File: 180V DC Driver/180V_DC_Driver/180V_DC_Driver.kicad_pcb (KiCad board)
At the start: 2 copper layers, 195 x 112 mm, 16 parts, among them J1 AC_In, J2 DC_Out, J3 Conn_01x02_Socket, J4 Conn_01x01_Socket, Q1 IRFP460PBF

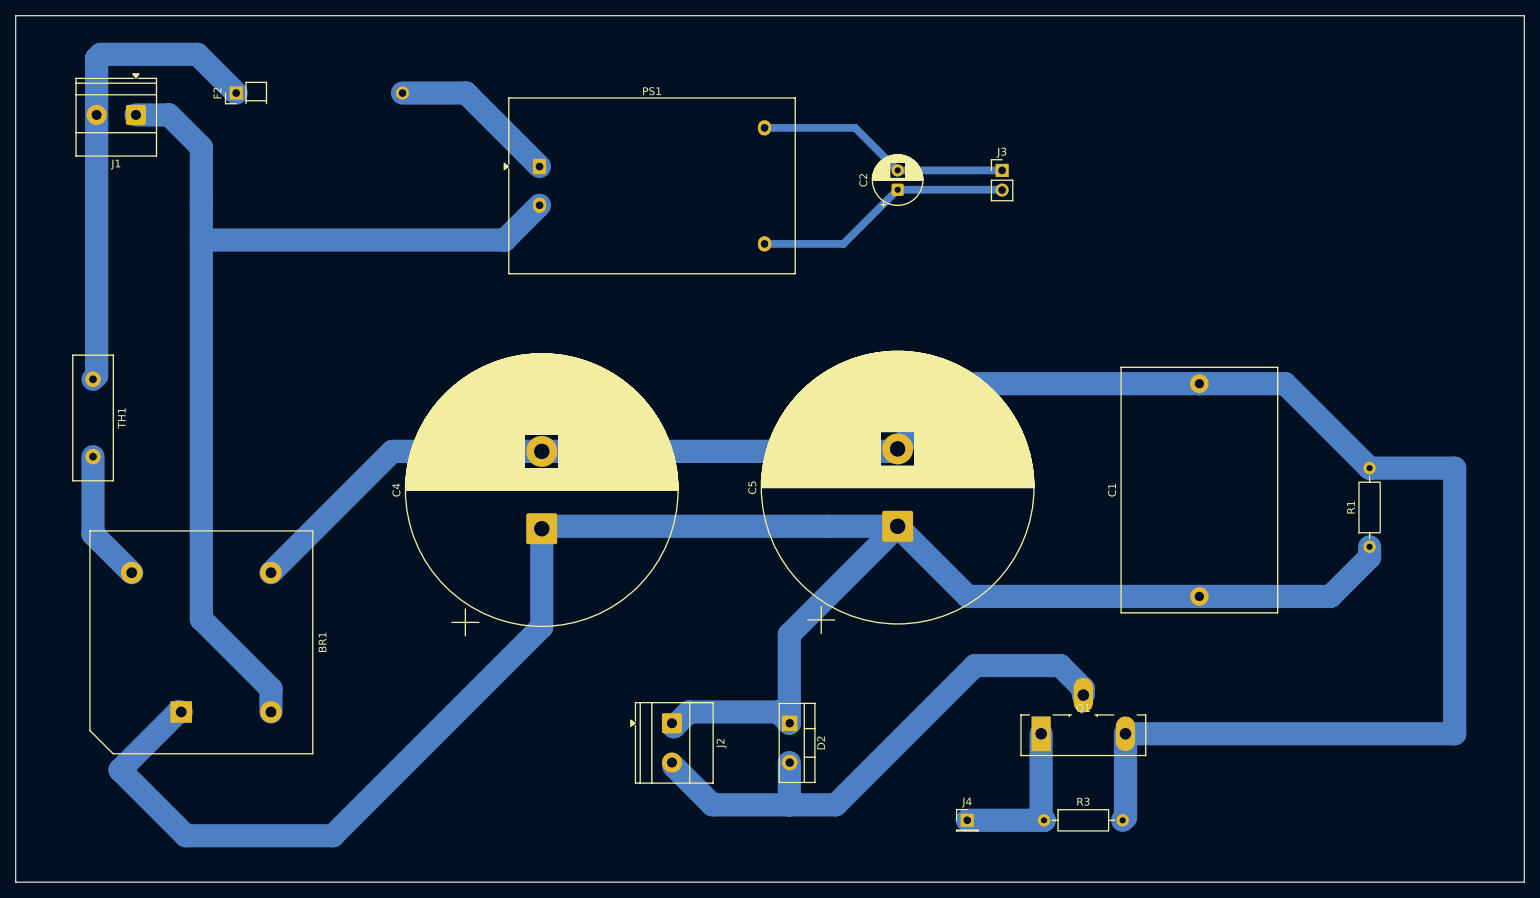
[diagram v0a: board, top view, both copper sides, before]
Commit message: c1806
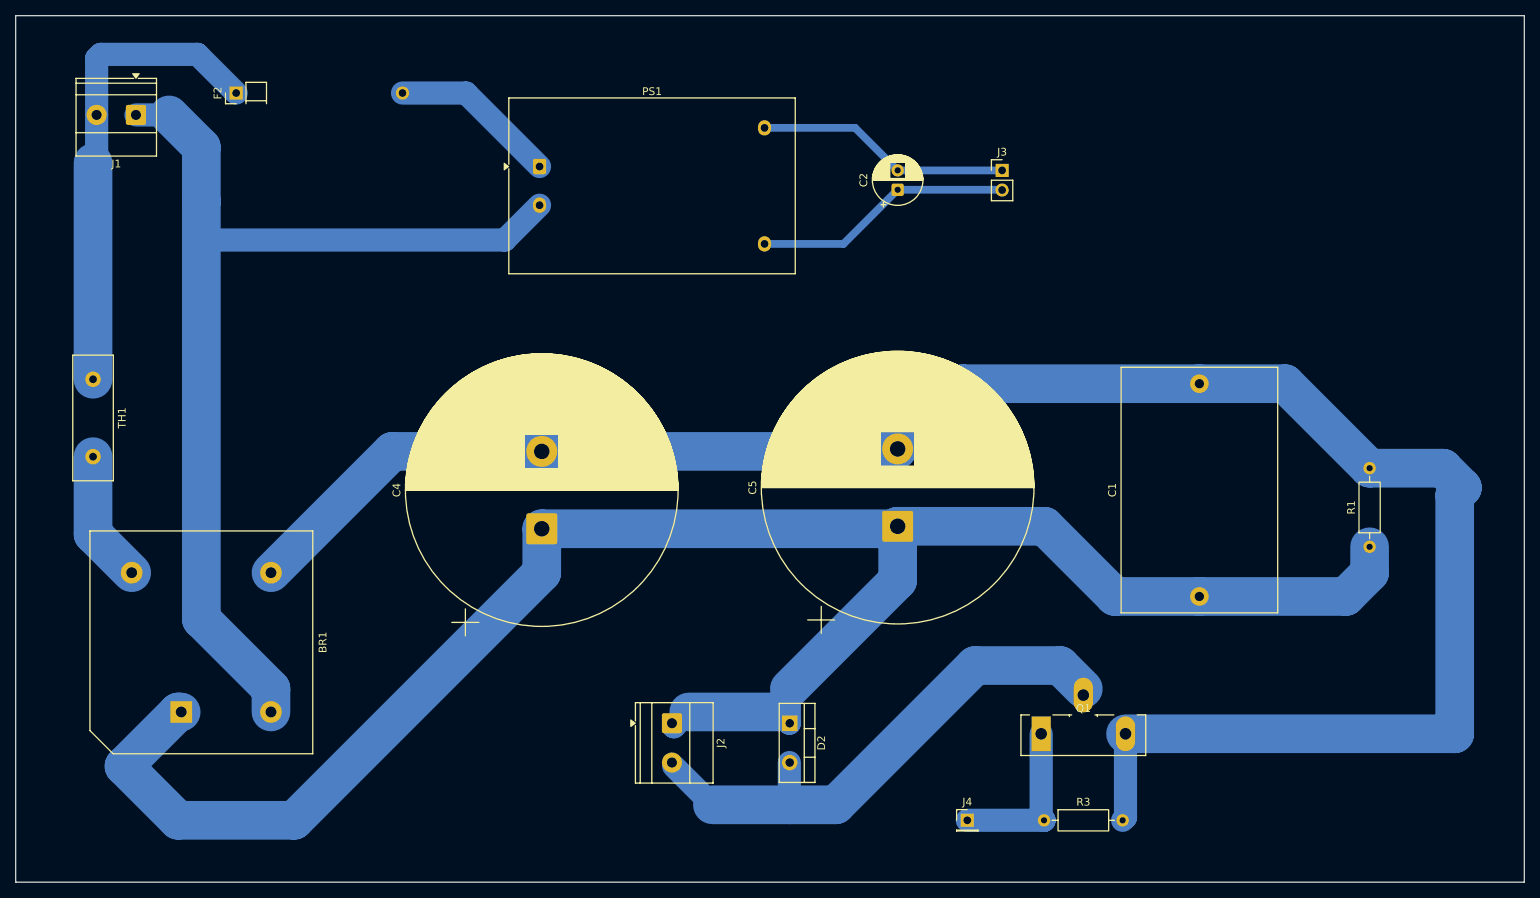
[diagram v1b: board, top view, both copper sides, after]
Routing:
- net Net-(BR1-+): track 254.8 -> 249.2 mm
